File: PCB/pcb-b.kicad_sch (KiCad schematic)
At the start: 11 parts, among them U1 L7805, U2 L7805, U3 L7805

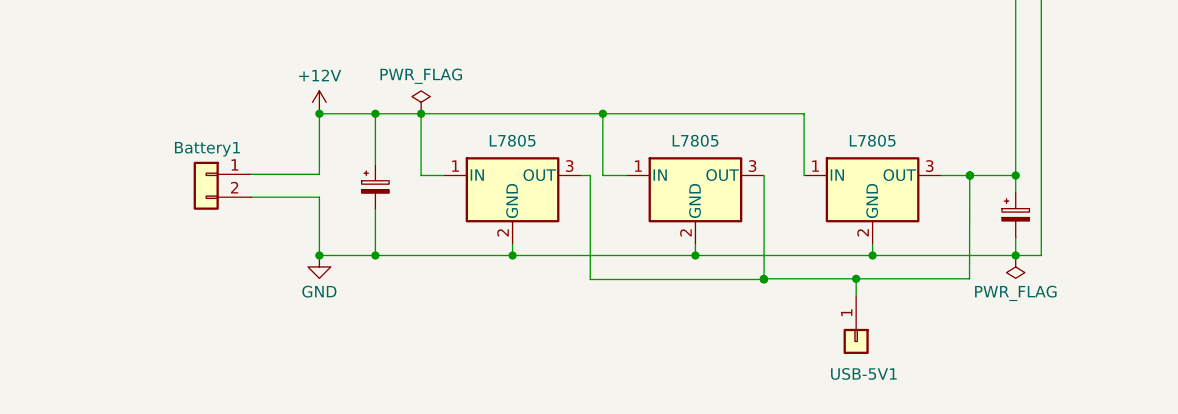
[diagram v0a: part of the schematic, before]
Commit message: fixes
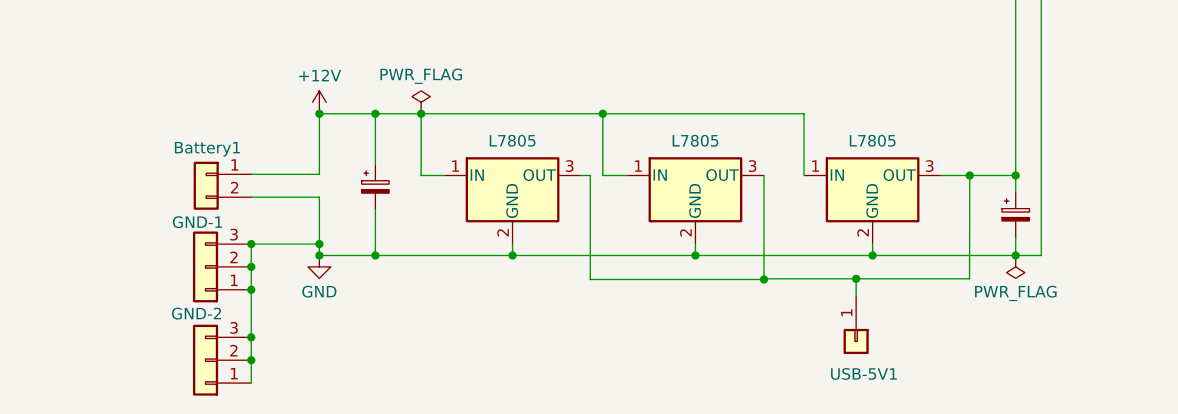
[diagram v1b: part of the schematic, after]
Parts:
- added GND-1, GND-2: ~, Connector_Wire:SolderWire-1.5sqmm_1x03_P6mm_D1.7mm_OD3mm, symbol Connector_Generic:Conn_01x03
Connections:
- net GND: now also GND-1.1 (Pin_1), GND-1.2 (Pin_2), GND-1.3 (Pin_3), GND-2.1 (Pin_1), GND-2.2 (Pin_2), GND-2.3 (Pin_3)
